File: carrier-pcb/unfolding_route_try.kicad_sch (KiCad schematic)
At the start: 66 parts, among them J1 USB_C_Receptacle_USB2.0, J2 Conn_01x04_Female, J3 1-338068-8, U1 TCA9548APWR, U10 DRV2605LDGS, U11 DRV2605LDGS, U12 BMX160, U2 TCA9548APWR, U3 DRV2605LDGS, U4 DRV2605LDGS, U5 DRV2605LDGS, U6 DRV2605LDGS, U7 DRV2605LDGS, U8 DRV2605LDGS, U9 DRV2605LDGS

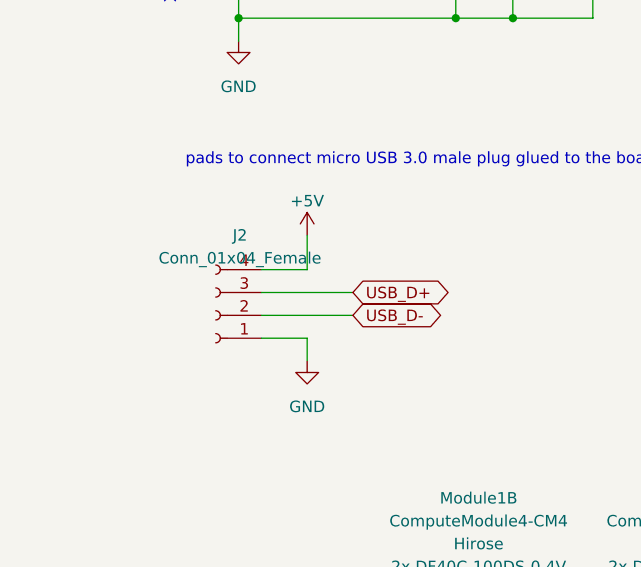
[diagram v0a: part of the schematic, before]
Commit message: New routing
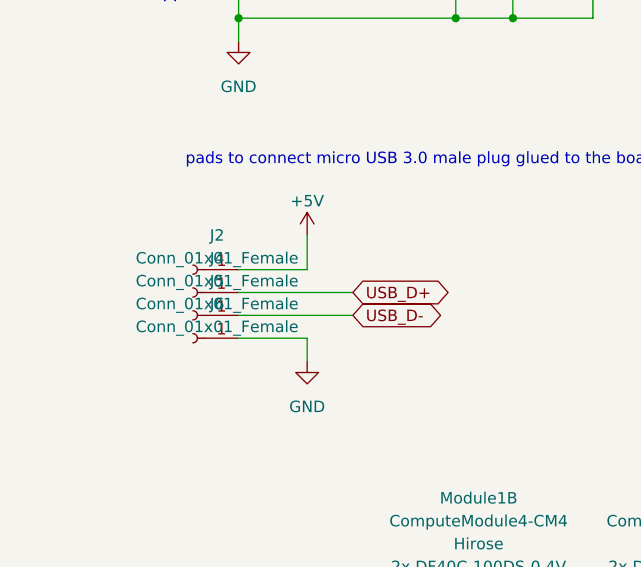
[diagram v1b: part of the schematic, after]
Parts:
- removed J2: Conn_01x04_Female, Connector_Wire:SolderWire-0.1sqmm_1x04_P3.6mm_D0.4mm_OD1mm, symbol Connector:Conn_01x04_Female
- added J2, J4, J5, J6: Conn_01x01_Female, Connector_Wire:SolderWirePad_1x01_SMD_1x2mm, symbol Connector:Conn_01x01_Female
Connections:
- net +5V: now also J2.1 (Pin_1)
- net GND: now also J6.1 (Pin_1)
- net USB_D+: now also J4.1 (Pin_1)
- net USB_D-: now also J5.1 (Pin_1)
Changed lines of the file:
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@@
     (stroke (width 0) (type solid) (color 0 0 0 0))
   )
-  (wire (pts (xy 38.1 99.06) (xy 43.18 99.06))
+  (wire (pts (xy 35.56 99.06) (xy 43.18 99.06))
     (stroke (width 0) (type solid) (color 0 0 0 0))
   )
-  (wire (pts (xy 38.1 101.6) (xy 48.26 101.6))
+  (wire (pts (xy 35.56 101.6) (xy 48.26 101.6))
     (stroke (width 0) (type solid) (color 0 0 0 0))
   )
-  (wire (pts (xy 38.1 104.14) (xy 48.26 104.14))
+  (wire (pts (xy 35.56 104.14) (xy 48.26 104.14))
     (stroke (width 0) (type solid) (color 0 0 0 0))
   )
-  (wire (pts (xy 38.1 106.68) (xy 43.18 106.68))
+  (wire (pts (xy 35.56 106.68) (xy 43.18 106.68))
     (stroke (width 0) (type solid) (color 0 0 0 0))
   )
@@
     (pin "1")
   )
+  (symbol (lib_id "Connector:Conn_01x01_Female") (at 30.48 99.06 180) (unit 1)
+    (in_bom yes) (on_board yes) (fields_autoplaced)
+    (property "Reference" "J2" (id 0) (at 33.1724 95.25 0))
+    (property "Value" "Conn_01x01_Female" (id 1) (at 33.1724 97.79 0))
+    (property "Footprint" "Connector_Wire:SolderWirePad_1x01_SMD_1x2mm" (id 2) (at 30.48 99.06 0)
+      (effects (font (size 1.27 1.27)) hide)
+    )
+    (property "Datasheet" "~" (id 3) (at 30.48 99.06 0)
+      (effects (font (size 1.27 1.27)) hide)
+    )
+    (pin "1")
+  )
+  (symbol (lib_id "Connector:Conn_01x01_Female") (at 30.48 101.6 180) (unit 1)
+    (in_bom yes) (on_board yes) (fields_autoplaced)
+    (property "Reference" "J4" (id 0) (at 33.1724 97.79 0))
+    (property "Value" "Conn_01x01_Female" (id 1) (at 33.1724 100.33 0))
+    (property "Footprint" "Connector_Wire:SolderWirePad_1x01_SMD_1x2mm" (id 2) (at 30.48 101.6 0)
+      (effects (font (size 1.27 1.27)) hide)
+    )
+    (property "Datasheet" "~" (id 3) (at 30.48 101.6 0)
+      (effects (font (size 1.27 1.27)) hide)
+    )
+    (pin "1")
+  )
+  (symbol (lib_id "Connector:Conn_01x01_Female") (at 30.48 104.14 180) (unit 1)
+    (in_bom yes) (on_board yes) (fields_autoplaced)
+    (property "Reference" "J5" (id 0) (at 33.1724 100.33 0))
+    (property "Value" "Conn_01x01_Female" (id 1) (at 33.1724 102.87 0))
+    (property "Footprint" "Connector_Wire:SolderWirePad_1x01_SMD_1x2mm" (id 2) (at 30.48 104.14 0)
+      (effects (font (size 1.27 1.27)) hide)
+    )
+    (property "Datasheet" "~" (id 3) (at 30.48 104.14 0)
+      (effects (font (size 1.27 1.27)) hide)
+    )
+    (pin "1")
+  )
+  (symbol (lib_id "Connector:Conn_01x01_Female") (at 30.48 106.68 180) (unit 1)
+    (in_bom yes) (on_board yes) (fields_autoplaced)
+    (property "Reference" "J6" (id 0) (at 33.1724 102.87 0))
+    (property "Value" "Conn_01x01_Female" (id 1) (at 33.1724 105.41 0))
+    (property "Footprint" "Connector_Wire:SolderWirePad_1x01_SMD_1x2mm" (id 2) (at 30.48 106.68 0)
+      (effects (font (size 1.27 1.27)) hide)
+    )
+    (property "Datasheet" "~" (id 3) (at 30.48 106.68 0)
+      (effects (font (size 1.27 1.27)) hide)
+    )
+    (pin "1")
+  )
   (symbol (lib_id "power:GND") (at 30.48 266.7 0) (unit 1)
     (in_bom yes) (on_board yes)
@@
     (pin "2")
   )
-  (symbol (lib_id "Connector:Conn_01x04_Female") (at 33.02 104.14 180) (unit 1)
-    (in_bom yes) (on_board yes) (fields_autoplaced)
-    (property "Reference" "J2" (id 0) (at 35.7124 95.25 0))
-    (property "Value" "Conn_01x04_Female" (id 1) (at 35.7124 97.79 0))
-    (property "Footprint" "Connector_Wire:SolderWire-0.1sqmm_1x04_P3.6mm_D0.4mm_OD1mm" (id 2) (at 33.02 104.14 0)
-      (effects (font (size 1.27 1.27)) hide)
-    )
-    (property "Datasheet" "~" (id 3) (at 33.02 104.14 0)
-      (effects (font (size 1.27 1.27)) hide)
-    )
-    (pin "1")
-    (pin "2")
-    (pin "3")
-    (pin "4")
-  )
   (symbol (lib_id "pspice:DIODE") (at 74.93 50.8 90) (unit 1)
     (in_bom yes) (on_board yes) (fields_autoplaced)
@@
       (reference "J1") (unit 1) (value "USB_C_Receptacle_USB2.0") (footprint "Connector_USB:USB_C_Receptacle_HRO_TYPE-C-31-M-12")
     )
-    (path "/a6b2795c-5490-47a0-885f-80e194c7f0a5"
-      (reference "J2") (unit 1) (value "Conn_01x04_Female") (footprint "Connector_Wire:SolderWire-0.1sqmm_1x04_P3.6mm_D0.4mm_OD1mm")
+    (path "/ac49e00a-5ed5-4857-8006-1aed13ae61c1"
+      (reference "J2") (unit 1) (value "Conn_01x01_Female") (footprint "Connector_Wire:SolderWirePad_1x01_SMD_1x2mm")
     )
     (path "/5cf17887-f1ff-4a1a-8009-890a9f14e0e0"
       (reference "J3") (unit 1) (value "1-338068-8") (footprint "footprints:1-338068-8")
     )
+    (path "/4d8a46ed-41fd-4cd4-b602-075741d0d23f"
+      (reference "J4") (unit 1) (value "Conn_01x01_Female") (footprint "Connector_Wire:SolderWirePad_1x01_SMD_1x2mm")
+    )
+    (path "/b3db4dfd-ded3-43ed-88e3-9230a4007ffc"
+      (reference "J5") (unit 1) (value "Conn_01x01_Female") (footprint "Connector_Wire:SolderWirePad_1x01_SMD_1x2mm")
+    )
+    (path "/60bd3e5d-30af-4910-bdbe-ab68030b2837"
+      (reference "J6") (unit 1) (value "Conn_01x01_Female") (footprint "Connector_Wire:SolderWirePad_1x01_SMD_1x2mm")
+    )
     (path "/223c5957-c5cf-487a-a2a3-5023ac54cb65"
